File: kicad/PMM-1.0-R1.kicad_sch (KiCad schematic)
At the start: 3 parts

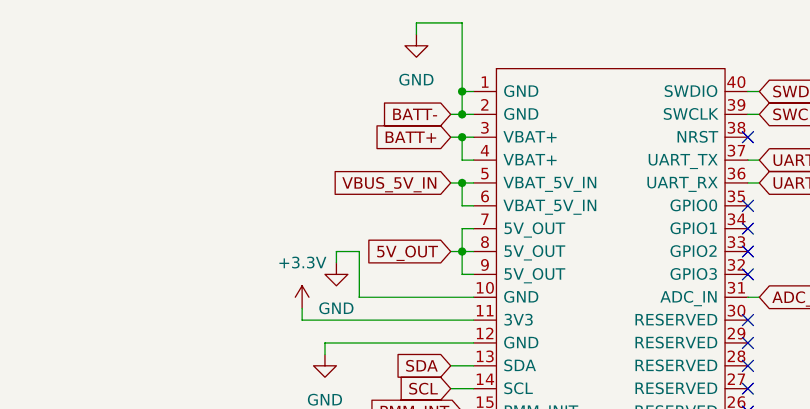
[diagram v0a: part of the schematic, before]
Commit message: start routing
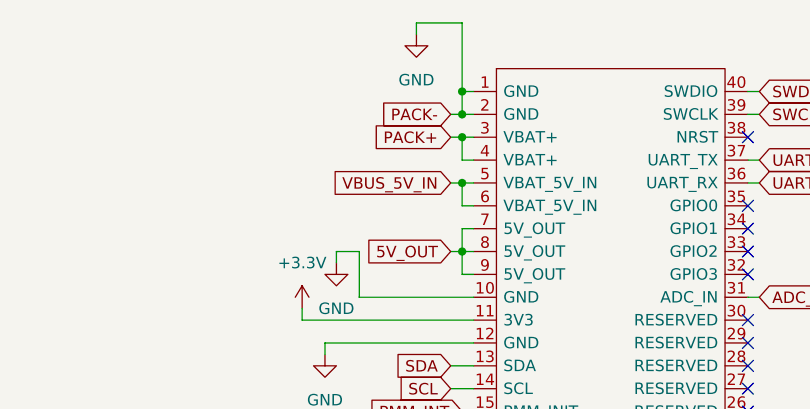
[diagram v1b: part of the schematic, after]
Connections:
- net BATT+ is gone; now on net PACK+: A1.3 (VBAT+), A1.4 (VBAT+)

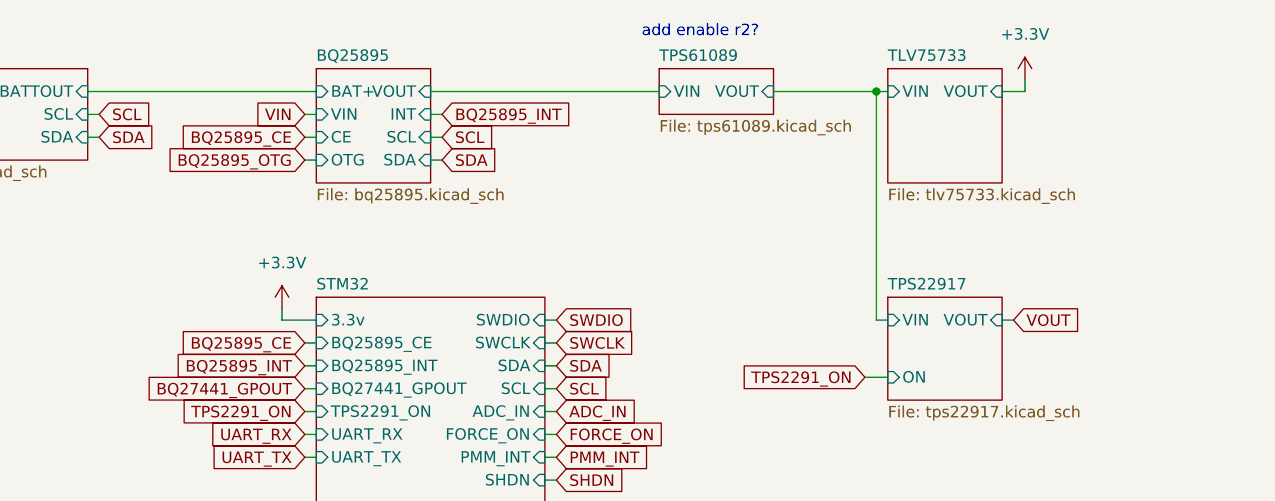
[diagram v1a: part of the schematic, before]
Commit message: finished pcb
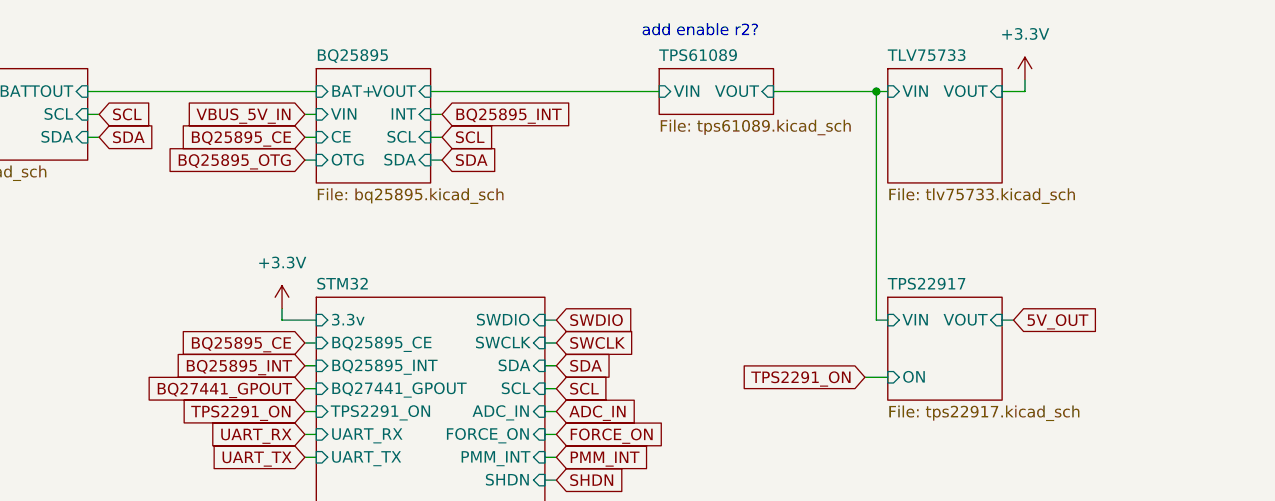
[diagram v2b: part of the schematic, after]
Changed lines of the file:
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@@
+		)
+	)
+	(global_label "5V_OUT"
+		(shape input)
+		(at 153.67 53.34 0)
+		(fields_autoplaced yes)
+		(effects
+			(font
+				(size 1.27 1.27)
+			)
+			(justify left)
+		)
+		(property "Intersheetrefs" "${INTERSHEET_REFS}"
+			(at 163.5495 53.34 0)
+			(hide yes)
+			(show_name no)
+			(do_not_autoplace no)
+			(effects
+				(font
+					(size 1.27 1.27)
+				)
+				(justify left)
+			)
 		)
 	)
@@
 		)
 	)
+	(global_label "VBUS_5V_IN"
+		(shape input)
+		(at 74.93 30.48 180)
+		(fields_autoplaced yes)
+		(effects
+			(font
+				(size 1.27 1.27)
+			)
+			(justify right)
+		)
+		(property "Intersheetrefs" "${INTERSHEET_REFS}"
+			(at 68.9209 30.48 0)
+			(hide yes)
+			(show_name no)
+			(do_not_autoplace no)
+			(effects
+				(font
+					(size 1.27 1.27)
+				)
+				(justify right)
+			)
+		)
+	)
 	(global_label "FORCE_ON"
 		(shape input)
@@
 			(hide yes)
 			(show_name no)
-			(do_not_autoplace no)
-			(effects
-				(font
-					(size 1.27 1.27)
-				)
-				(justify left)
-			)
-		)
-	)
-	(global_label "VIN"
-		(shape input)
-		(at 74.93 30.48 180)
-		(fields_autoplaced yes)
-		(effects
-			(font
-				(size 1.27 1.27)
-			)
-			(justify right)
-		)
-		(property "Intersheetrefs" "${INTERSHEET_REFS}"
-			(at 68.9209 30.48 0)
-			(hide yes)
-			(show_name no)
-			(do_not_autoplace no)
-			(effects
-				(font
-					(size 1.27 1.27)
-				)
-				(justify right)
-			)
-		)
-	)
-	(global_label "VOUT"
-		(shape input)
-		(at 153.67 53.34 0)
-		(fields_autoplaced yes)
-		(effects
-			(font
-				(size 1.27 1.27)
-			)
-			(justify left)
-		)
-		(property "Intersheetrefs" "${INTERSHEET_REFS}"
-			(at 161.3724 53.34 0)
-			(hide yes)
-			(show_name no)
